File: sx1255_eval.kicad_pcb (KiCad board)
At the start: 2 copper layers, 43 x 34 mm, 28 parts, among them IC1 SX1255, J1 EXT_CLK_IN, J2 TX_SMA, J3 RX_SMA, J4 CONN

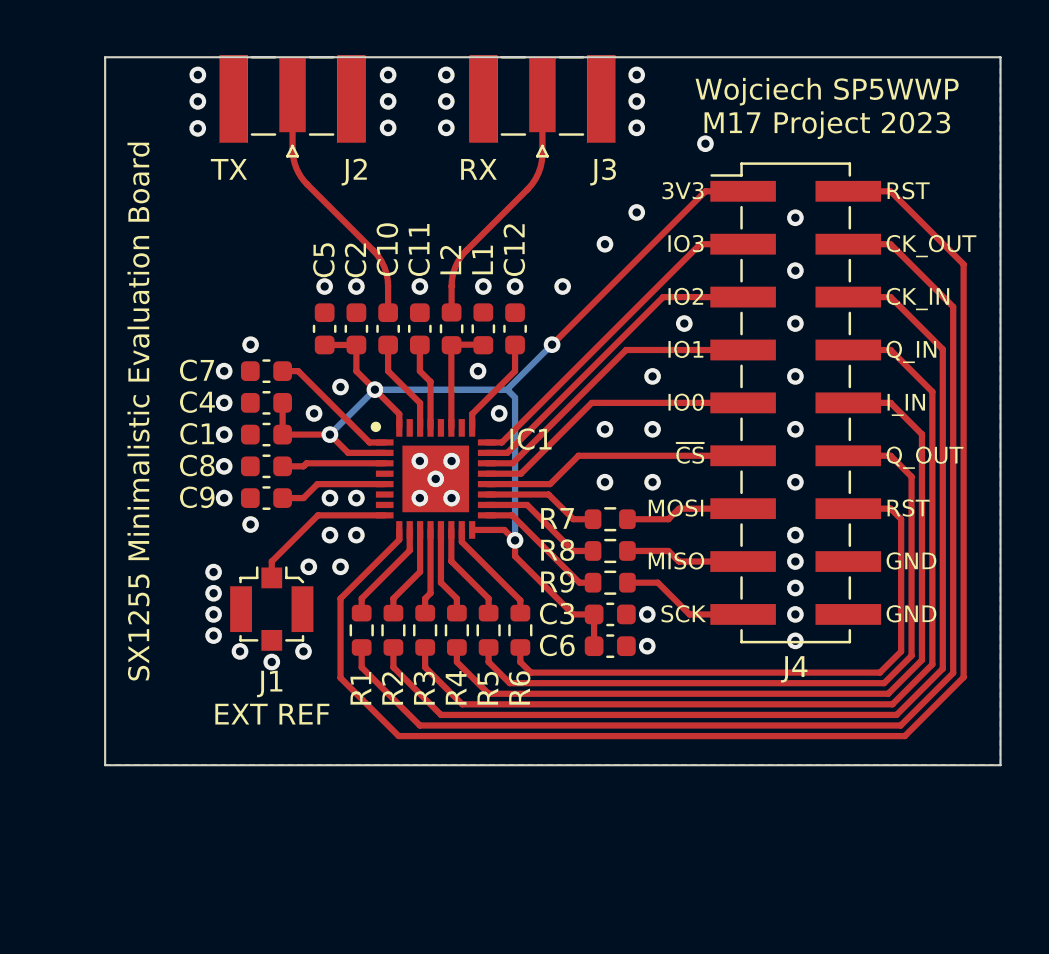
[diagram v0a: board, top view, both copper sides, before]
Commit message: PMOD
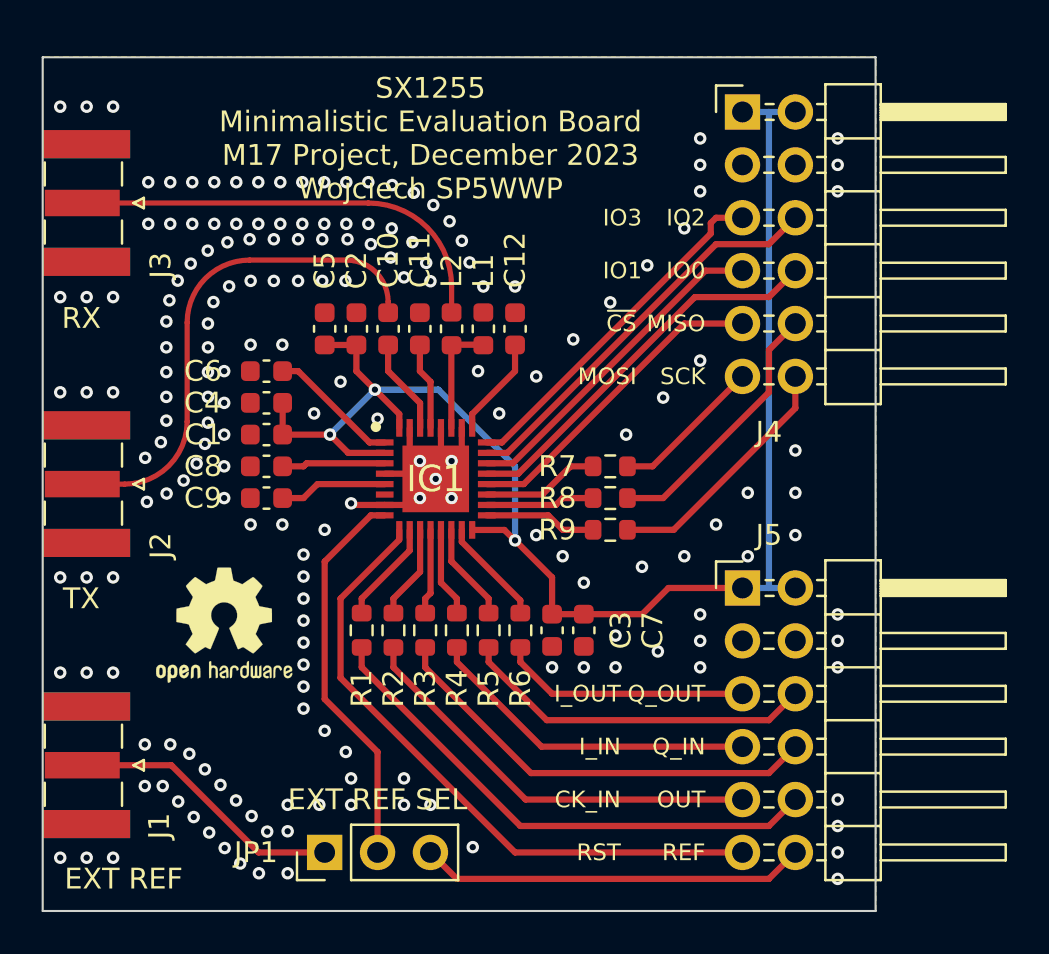
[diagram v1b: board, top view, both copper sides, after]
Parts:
- added J5: PMOD, Connector_PinHeader_2.54mm:PinHeader_2x06_P2.54mm_Horizontal, F.Cu at (165.6, 94.5)
- added JP1: EXT_CLK_SRC, Connector_PinHeader_2.54mm:PinHeader_1x03_P2.54mm_Vertical, F.Cu at (145.5, 107.2)
- added REF**: OSHW-Logo2_7.3x6mm_SilkScreen, Symbol:OSHW-Logo2_7.3x6mm_SilkScreen, F.Cu at (140.7, 96.3)
- J1: footprint Connector_Coaxial:U.FL_Molex_MCRF_73412-0110_Vertical -> Connector_Coaxial:SMA_Samtec_SMA-J-P-X-ST-EM1_EdgeMount
- J4: value CONN -> PMOD; footprint Connector_PinHeader_2.54mm:PinHeader_2x09_P2.54mm_Vertical_SMD -> Connector_PinHeader_2.54mm:PinHeader_2x06_P2.54mm_Horizontal
- moved J3 22.5 mm to (134.1, 76.0), turned to -90 degrees
- moved J2 21.0 mm to (134.1, 89.5), turned to -90 degrees
- moved J4 14.2 mm to (165.6, 71.6)
- moved J1 11.6 mm to (134.1, 103.0), turned to -90 degrees
- moved C3 2.90 mm to (156.5, 96.5), turned to -90 degrees
- moved R7 2.54 mm to (159.3, 88.6)
- moved R8 2.54 mm to (159.3, 90.2)
- moved R9 2.54 mm to (159.3, 91.7)
- moved C7 1.48 mm to (158.0, 96.5), turned to -90 degrees
- renumbered C7 to C6, C6 to C7
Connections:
- net Net-(J2-In) renamed /RF_OUT
- net Net-(J3-In) renamed /RF_IN
- J1 pad 1: EXT_CLK -> EXT_CLK_B
- J4 pad 10: I_IN -> MISO
- J4 pad 11: ~{CS} -> MOSI
- J4 pad 12: Q_OUT -> SCK
- J4 pad 2: RST -> +3V3
- J4 pad 3: DIO3 -> GND
- J4 pad 4: CK_OUT -> GND
- J4 pad 5: DIO2 -> DIO3
- J4 pad 6: CK_IN -> DIO2
- J4 pad 8: Q_IN -> DIO0
- J4 pad 9: DIO0 -> ~{CS}
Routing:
- net RST: track 67.4 -> 31.1 mm
- net CK_OUT: track 55.4 -> 25.5 mm
- net CK_IN: track 50.1 -> 20.3 mm
- net Q_IN: track 44.8 -> 21.4 mm
- net I_IN: track 39.3 -> 16.1 mm
- net EXT_CLK_A: track 0.00 -> 18.6 mm
- net +3V3: track 54.7 -> 72.2 mm, vias 4 -> 3
- net Q_OUT: track 34.0 -> 17.1 mm
- net I_OUT: track 28.7 -> 12.0 mm
- net EXT_CLK_B: track 0.00 -> 13.4 mm
- net GND: track 0.00 -> 12.2 mm, vias 69 -> 186
- net /RF_OUT: track 12.1 -> 24.2 mm
- net EXT_CLK: track 7.13 -> 18.8 mm
- net /RF_IN: track 12.0 -> 21.1 mm
- net MISO: track 5.77 -> 12.7 mm
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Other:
- board size 43 x 34 mm -> 40 x 41 mm
- board text added: "EXT REF SEL"
- board text added: "I_OUT"
- board text added: "OUT"
- board text added: "REF"
- board text added: "SX1255 Minimalistic Evaluation Board M17 Project, December 2023 Wojciech SP5WWP"
- board text removed: "3V3"
- board text removed: "CK_OUT"
- board text removed: "GND"
- board text removed: "SX1255 Minimalistic Evaluation Board"
- board text removed: "Wojciech SP5WWP M17 Project 2023"
